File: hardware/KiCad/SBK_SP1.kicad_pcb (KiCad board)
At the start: 2 copper layers, 10.7 x 11.1 mm, 10 parts, among them J1 1x4 pin header, Q1 AO3400A, Q2 AO3401A

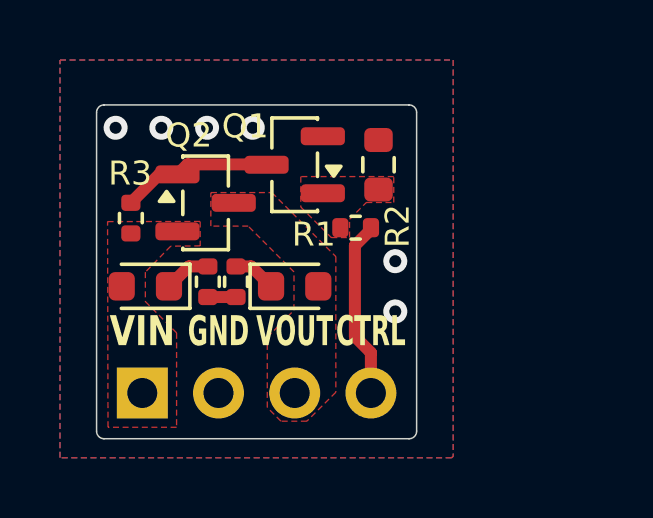
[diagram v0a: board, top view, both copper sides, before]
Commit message: SBK_SP1 V2..0 updates
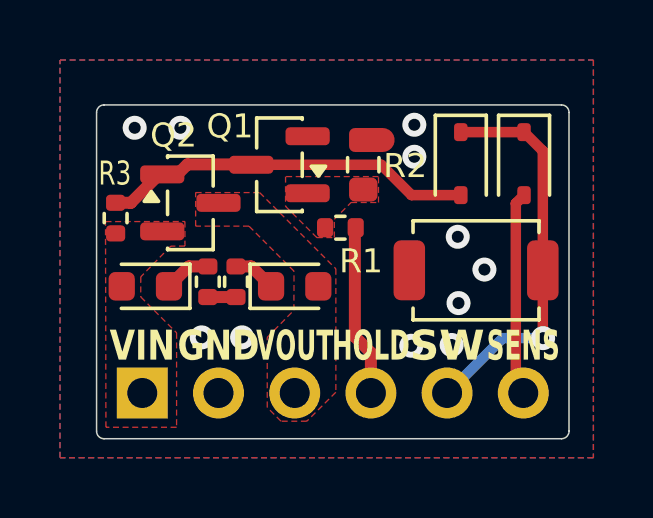
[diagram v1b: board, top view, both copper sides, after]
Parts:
- added D3: 1N4148, Diode_SMD:D_SOD-323, F.Cu at (124.9, 81.3)
- added D4: 1N4148, Diode_SMD:D_SOD-323, F.Cu at (127.0, 81.3)
- added SW1: TS-1088-AR02016, Button_Switch_SMD:SW_SPST_TS-1088-xR020, F.Cu at (125.4, 84.8)
- J1: value 1x4 pin header -> Conn_01x06; footprint Connector_PinHeader_2.54mm:PinHeader_1x04_P2.54mm_Vertical -> Connector_PinHeader_2.54mm:PinHeader_1x06_P2.54mm_Vertical
- moved R2 0.51 mm to (121.7, 81.3)
- moved Q1 0.51 mm to (118.9, 81.3)
- moved Q2 0.51 mm to (115.9, 82.6)
- moved R1 0.51 mm to (120.9, 83.4)
- moved R3 0.51 mm to (113.4, 83.1)
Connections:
- net CTRL renamed Net-(J1-Pin_4)
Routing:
- net Net-(D3-K): track 0.00 -> 13.2 mm, vias 0 -> 1
- net Net-(D4-A): track 0.00 -> 6.81 mm
- net Net-(D3-A): track 5.06 -> 11.8 mm
- net GND: track 0.94 -> 1.59 mm, vias 6 -> 11
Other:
- board size 10.7 x 11.1 mm -> 15.7 x 11.1 mm
- board text added: "HOLD"
- board text added: "SBK_SP1 v2.0"
- board text added: "SENS"
- board text added: "SW"
- board text added: "VIN 2-12V MAX LOAD 2A HOLD HIGH = ON START: BTN / SW -> GND"
- board text removed: "CTRL"
- board text removed: "SBK_SP1 v1.0"
- board text removed: "VIN 2-12V MAX LOAD 2A CTRL 0-VIN"
